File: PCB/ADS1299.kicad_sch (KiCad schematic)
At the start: 36 parts, among them CN1 W2A41C681KAT2A, CN2 W2A41C681KAT2A, CN3 W2A41C681KAT2A, CN4 W2A41C681KAT2A, U1 ADS1299IPAGR, U3 TPD4E1B06DCKR, U4 TPD4E1B06DCKR, U9 TPD4E1B06DCKR

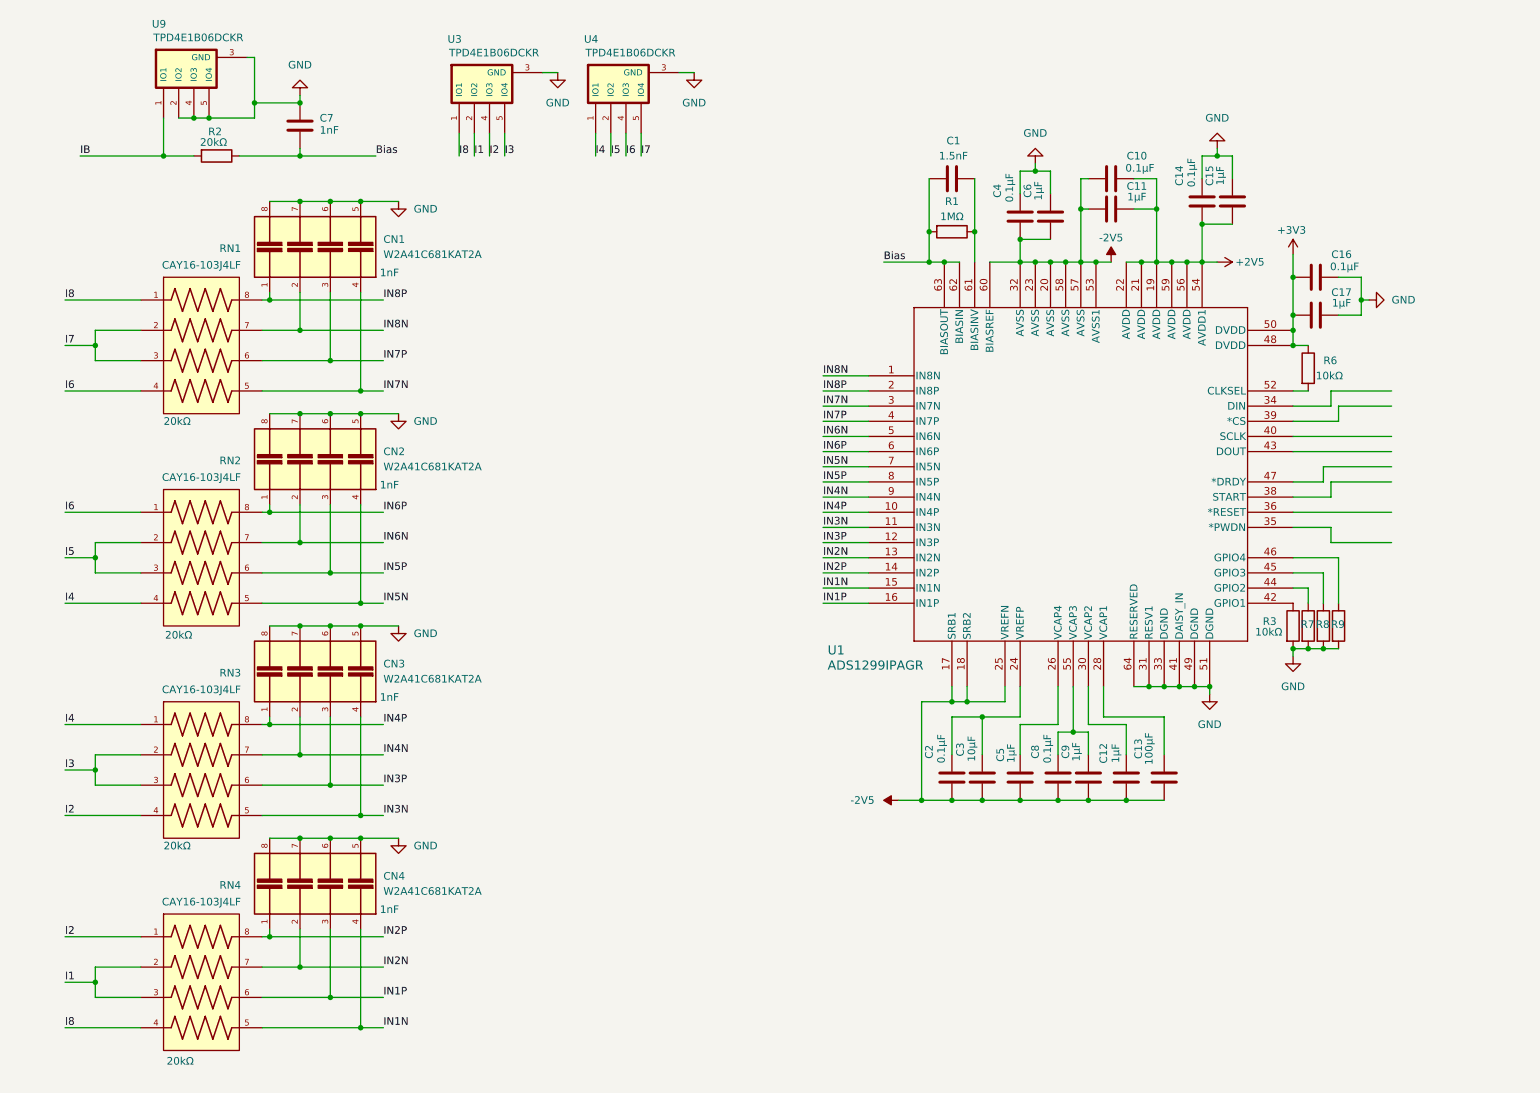
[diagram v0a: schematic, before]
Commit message: ads1299 sheet
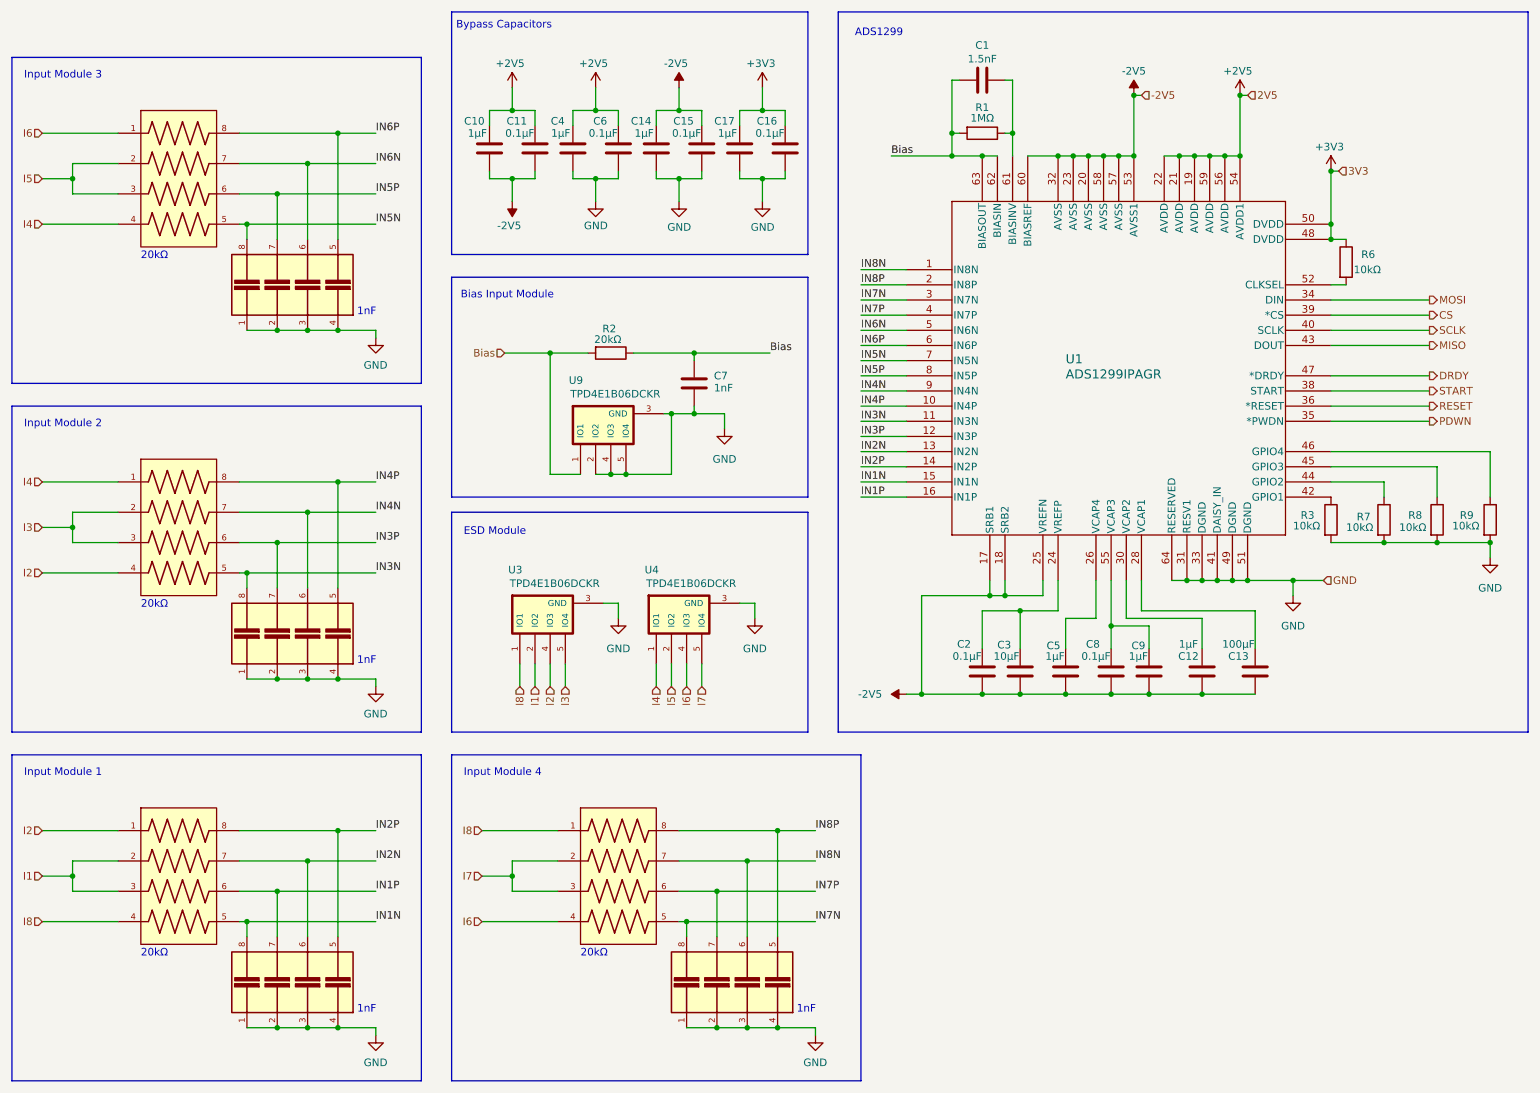
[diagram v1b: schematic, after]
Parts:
- removed CN1, CN3, CN4: W2A41C681KAT2A, W2A41C681KAT2A:CAPCAXE50P210X130X94-8N, symbol custom_lib:W2A41C681KAT2A
- removed RN1, RN2, RN3, RN4: CAY16-103J4LF, CAY16-103J4LF:RESCAF80P320X160X60-8N, symbol custom_lib:CAY16-103J4LF
- added CN5, CN6, CN7: W2A41C681KAT2A, W2A41C681KAT2A:CAPCAXE50P210X130X94-8N, symbol custom_lib:W2A41C681KAT2A
- added RN5, RN6, RN7, RN8: CAY16-103J4LF, CAY16-103J4LF:RESCAF80P320X160X60-8N, symbol custom_lib:CAY16-103J4LF
- C10, C14, C4: value 0.1µF -> 1µF
- C11, C15, C6: value 1µF -> 0.1µF
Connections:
- net IB is gone; now on net Bias: R2.2, U9.1 (IO1)
- net +2V5: now also C10.1, C11.1, C4.1, C6.1; no longer C10.2, C11.2, C14.1, C15.1
- net -2V5: now also C10.2, C11.2, C14.1, C15.1; no longer C10.1, C11.1, C4.1, C6.1
- net Bias: now also C7.1; no longer C7.2
- net GND: now also C7.2, CN2.1, CN2.2, CN2.3, CN2.4, CN5.1, CN5.2, CN5.3, CN5.4, CN6.1, CN6.2, CN6.3, CN6.4, CN7.1, CN7.2, CN7.3, CN7.4; no longer C7.1, CN2.5, CN2.6, CN2.7, CN2.8
- net I1: now also RN8.2, RN8.3
- net I2: now also RN7.4, RN8.1
- net I3: now also RN7.2, RN7.3
- net I4: now also RN6.4, RN7.1
- net I5: now also RN6.2, RN6.3
- net I6: now also RN5.4, RN6.1
- net I7: now also RN5.2, RN5.3
- net I8: now also RN5.1, RN8.4
- net IN1N: now also CN7.8, RN8.5
- net IN1P: now also CN7.7, RN8.6
- net IN2N: now also CN7.6, RN8.7
- net IN2P: now also CN7.5, RN8.8
- net IN3N: now also CN6.8, RN7.5
- net IN3P: now also CN6.7, RN7.6
- net IN4N: now also CN6.6, RN7.7
- net IN4P: now also CN6.5, RN7.8
- net IN5N: now also CN5.8, RN6.5; no longer CN2.4
- net IN5P: now also CN5.7, RN6.6; no longer CN2.3
- net IN6N: now also CN5.6, RN6.7; no longer CN2.2
- net IN6P: now also CN5.5, RN6.8; no longer CN2.1
- net IN7N: now also CN2.8, RN5.5
- net IN7P: now also CN2.7, RN5.6
- net IN8N: now also CN2.6, RN5.7
- net IN8P: now also CN2.5, RN5.8
- net MOSI: now reaches U1.34 (DIN)
- net PDWN: now reaches U1.35 (*PWDN)
- net RESET: now reaches U1.36 (*RESET)
- net START: now reaches U1.38 (START)
- net CS: now reaches U1.39 (*CS)
- net SCLK: now reaches U1.40 (SCLK)
- net MISO: now reaches U1.43 (DOUT)
- net DRDY: now reaches U1.47 (*DRDY)
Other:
- note added: "ADS1299"
- note added: "Bias Input Module"
- note added: "Bypass Capacitors"
- note added: "ESD Module"
- note added: "Input Module 1"
- note added: "Input Module 2"
- note added: "Input Module 3"
- note added: "Input Module 4"
- moved on the sheet: C1, C12, C13, C2, C3, C5, C8, C9, R1, R3, R6, R7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
